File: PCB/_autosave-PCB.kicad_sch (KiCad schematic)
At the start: 148 parts, among them J1 USB_C_Receptacle_USB2.0_16P, J2 Battery, J3 Conn_01x04, J4 Conn_01x05, Q1 AO3401A, Q2 2N7002, Q3 2N7002, SW1 SW_Push, SW10 MX_SW_HS, SW11 MX_SW_HS, SW12 MX_SW_HS, SW13 MX_SW_HS, SW14 MX_SW_HS, SW15 MX_SW_HS, SW16 MX_SW_HS, SW17 MX_SW_HS, SW18 MX_SW_HS, SW19 MX_SW_HS, SW2 MX_SW_HS, SW20 MX_SW_HS, SW21 MX_SW_HS, SW22 MX_SW_HS, SW23 MX_SW_HS, SW24 MX_SW_HS, SW25 MX_SW_HS, SW26 MX_SW_HS, SW27 MX_SW_HS, SW28 MX_SW_HS, SW29 MX_SW_HS, SW3 MX_SW_HS, SW30 SW_SPDT, SW31 MX_SW_HS, SW32 MX_SW_HS, SW33 MX_SW_HS, SW34 MX_SW_HS, SW35 MX_SW_HS, SW36 MX_SW_HS, SW37 MX_SW_HS, SW4 MX_SW_HS, SW5 MX_SW_HS, SW6 MX_SW_HS, SW7 MX_SW_HS, SW8 MX_SW_HS, SW9 MX_SW_HS, U1 MAX17048, U2 DW01A, U3 FS8205, U4 BQ24075RGT, U5 nRF52840_E73-2G4M08S1C, Y1 32.768 KHz

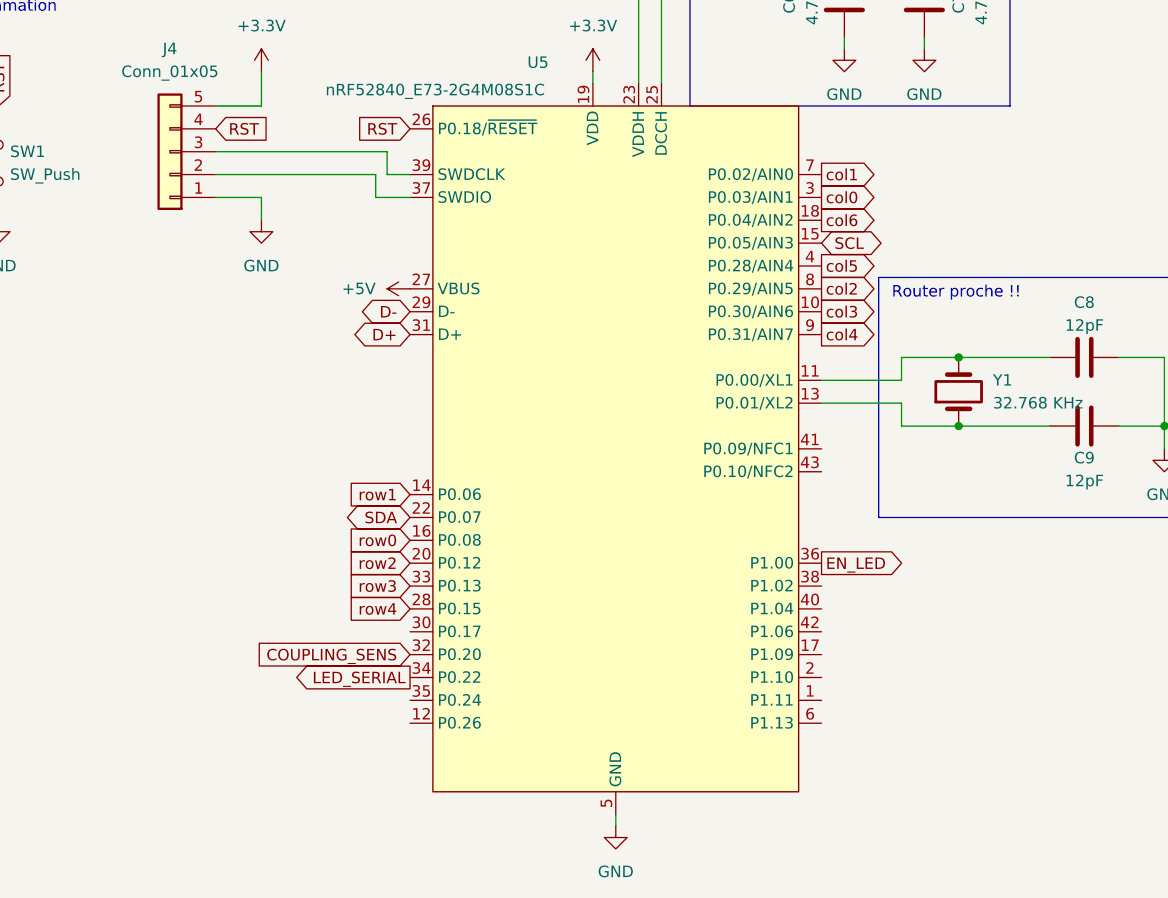
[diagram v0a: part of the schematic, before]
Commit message: Added circuit and started PCB
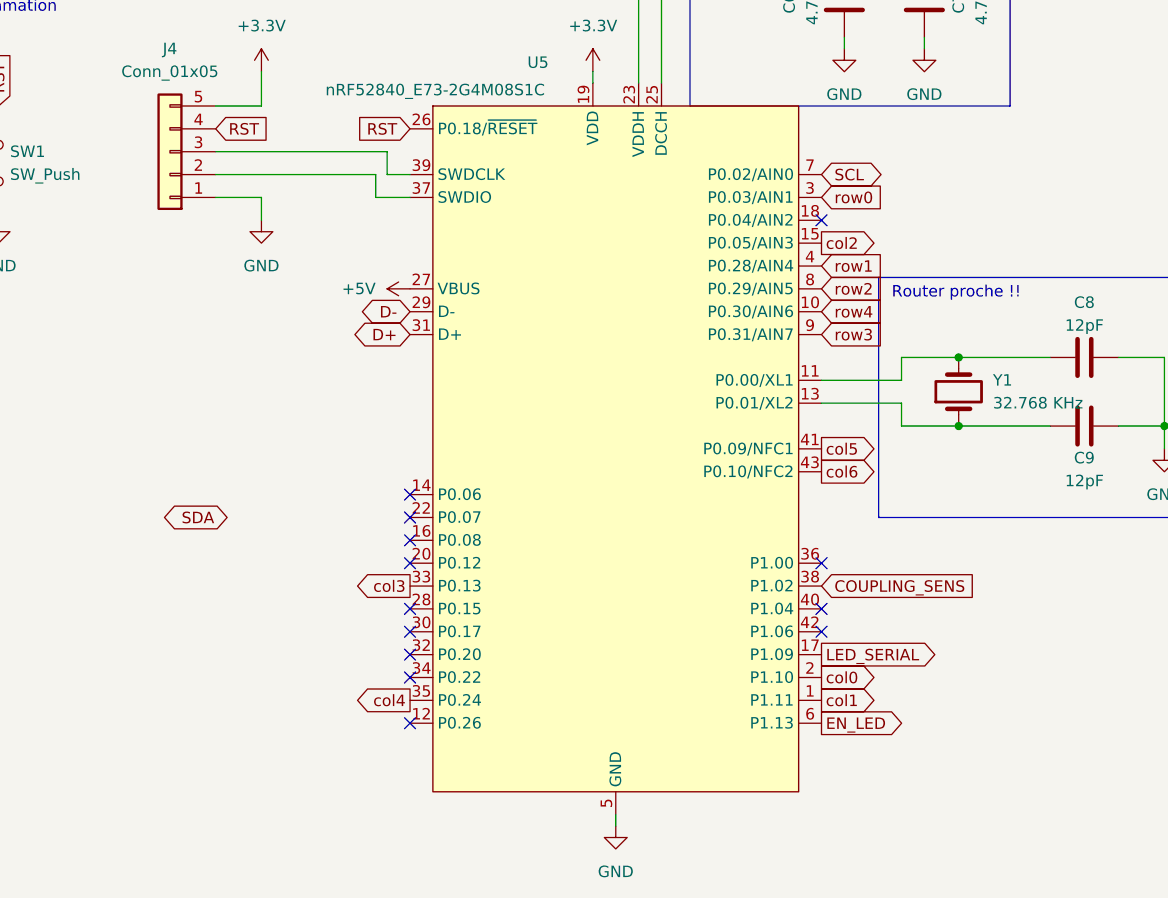
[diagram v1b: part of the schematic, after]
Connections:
- net COUPLING_SENS: now also U5.38 (P1.02); no longer U5.32 (P0.20)
- net EN_LED: now also U5.6 (P1.13); no longer U5.36 (P1.00)
- net LED_SERIAL: now also U5.17 (P1.09); no longer U5.34 (P0.22)
- net SCL: now also U5.7 (P0.02/AIN0); no longer U5.15 (P0.05/AIN3)
- net SDA: no longer U5.22 (P0.07)
- net col0: now also U5.2 (P1.10); no longer U5.3 (P0.03/AIN1)
- net col1: now also U5.1 (P1.11); no longer U5.7 (P0.02/AIN0)
- net col2: now also U5.15 (P0.05/AIN3); no longer U5.8 (P0.29/AIN5)
- net col3: now also U5.33 (P0.13); no longer U5.10 (P0.30/AIN6)
- net col4: now also U5.35 (P0.24); no longer U5.9 (P0.31/AIN7)
- net col5: now also U5.41 (P0.09/NFC1); no longer U5.4 (P0.28/AIN4)
- net col6: now also U5.43 (P0.10/NFC2); no longer U5.18 (P0.04/AIN2)
- net row0: now also U5.3 (P0.03/AIN1); no longer U5.16 (P0.08)
- net row1: now also U5.4 (P0.28/AIN4); no longer U5.14 (P0.06)
- net row2: now also U5.8 (P0.29/AIN5); no longer U5.20 (P0.12)
- net row3: now also U5.9 (P0.31/AIN7); no longer U5.33 (P0.13)
- net row4: now also U5.10 (P0.30/AIN6); no longer U5.28 (P0.15)
- no-connect marks 7 -> 20
